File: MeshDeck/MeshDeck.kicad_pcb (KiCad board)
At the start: 4 copper layers, 44 parts, among them CN1 ATGM336H-6N-74, SW1 4*4*1.7, SW2 4*4*1.7, U1 ESP32-S3-WROOM-1(N16R8), U2 SX1262S8S+T-X1, U3 TPS6282533DMQR, U4 BQ24074RGTR, U5 RN32768114

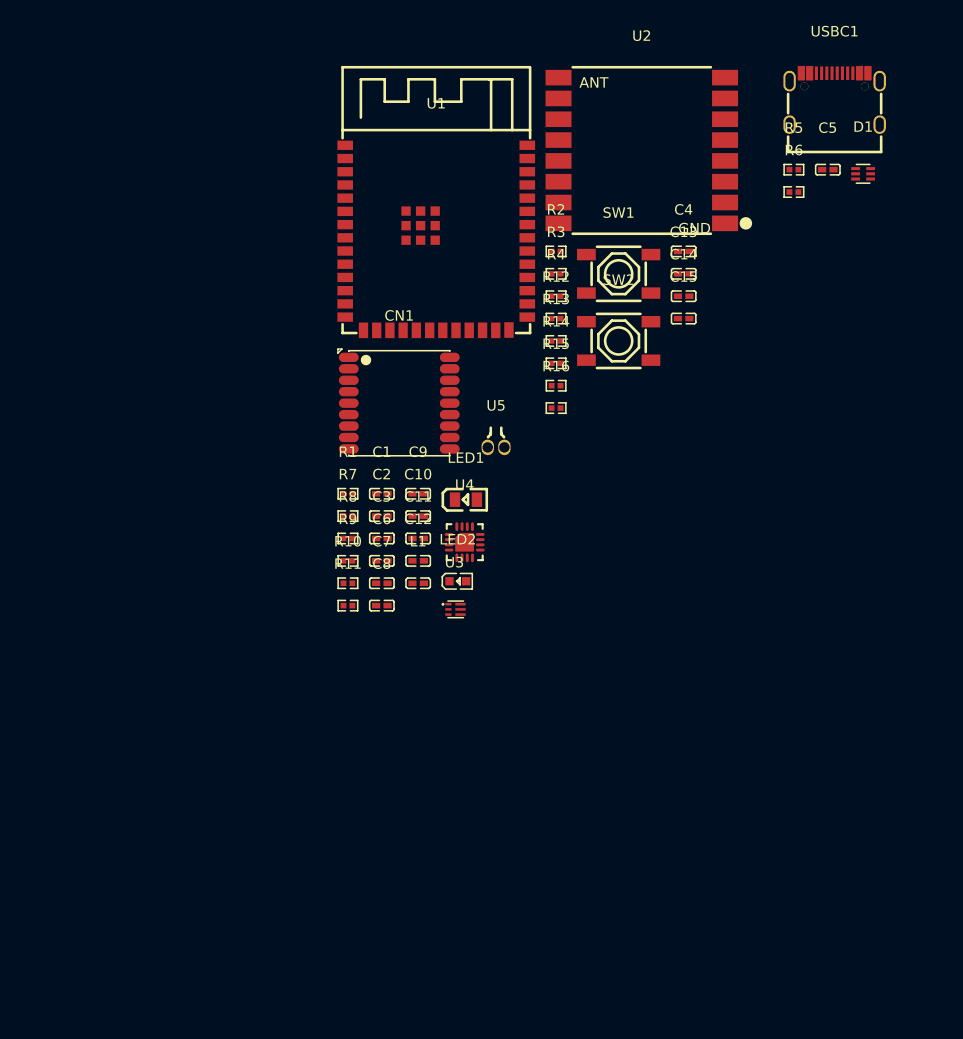
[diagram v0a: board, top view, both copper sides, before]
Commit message: set up LoRa module and screen (wip)
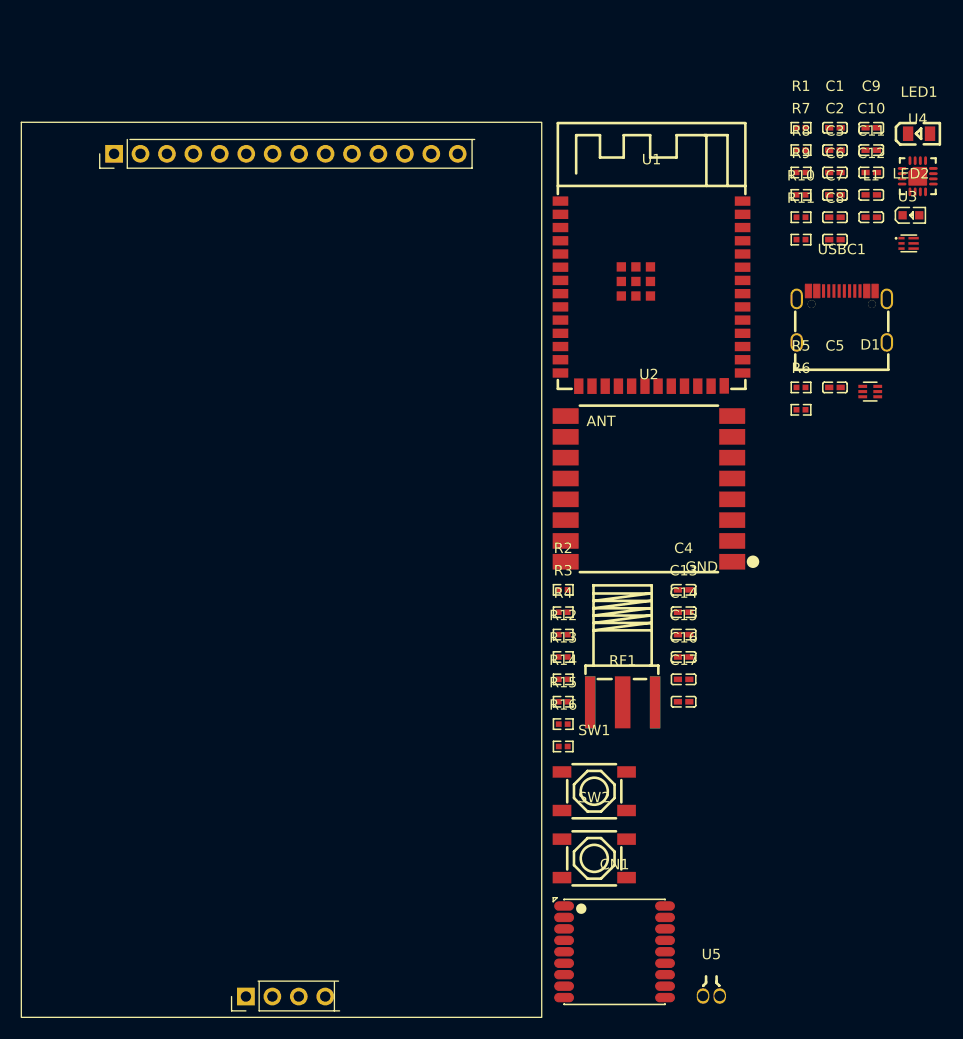
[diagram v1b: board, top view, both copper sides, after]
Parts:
- added C16: 1uF, MeshDeck:C0402, F.Cu at (153.0, 102.6)
- added C17: 1Nf, MeshDeck:C0402, F.Cu at (153.0, 104.7)
- added RF1: HJ-SMA023, MeshDeck:SMA-SMD_HJ-SMA023, F.Cu at (147.2, 104.8)
- added U6: ~, MeshDeck:2.8 SPI LCD TFT ST7789, F.Cu at (114.4, 69.3)
- moved U5 56.6 mm to (155.7, 133.0)
- moved CN1 56.6 mm to (146.4, 128.8)
- moved U3 56.0 mm to (174.6, 60.7)
- moved C11 56.0 mm to (171.1, 53.9)
- moved L1 56.0 mm to (171.1, 58.2)
- moved LED2 56.0 mm to (174.9, 58.0)
- moved R10 56.0 mm to (164.3, 58.2)
- moved R8 56.0 mm to (164.3, 53.9)
- moved U4 56.0 mm to (175.5, 54.2)
- moved C10 56.0 mm to (171.1, 51.7)
- moved C12 56.0 mm to (171.1, 56.0)
- moved C3 56.0 mm to (167.6, 53.9)
- moved C7 56.0 mm to (167.6, 58.2)
- moved C9 56.0 mm to (171.1, 49.6)
- moved LED1 56.0 mm to (175.7, 50.1)
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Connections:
- U1 pad 10: unconnected-(U1-IO17-Pad10) -> /IO17
- U1 pad 17: unconnected-(U1-IO9-Pad17) -> /IO9
- U1 pad 19: unconnected-(U1-IO11-Pad19) -> /IO11
- U1 pad 20: unconnected-(U1-IO12-Pad20) -> /IO12
- U1 pad 21: unconnected-(U1-IO13-Pad21) -> /IO13
- U1 pad 22: unconnected-(U1-IO14-Pad22) -> /IO14
- U1 pad 26: unconnected-(U1-IO45-Pad26) -> /IO45
- U1 pad 32: unconnected-(U1-IO39-Pad32) -> /SPI.SCK
- U1 pad 33: unconnected-(U1-IO40-Pad33) -> /SPI.MISO
- U1 pad 34: unconnected-(U1-IO41-Pad34) -> /SPI.MOSI
- U1 pad 35: unconnected-(U1-IO42-Pad35) -> /IO42
- U2 pad 1: unconnected-(U2-GND-Pad1) -> GND
- U2 pad 10: unconnected-(U2-GND-Pad10) -> GND
- U2 pad 11: unconnected-(U2-RXE-Pad11) -> /IO14
- U2 pad 13: unconnected-(U2-VCC-Pad13) -> /3V3
- U2 pad 15: unconnected-(U2-DIO1-Pad15) -> /IO45
- U2 pad 16: unconnected-(U2-BUSY-Pad16) -> /IO13
- U2 pad 2: unconnected-(U2-SO-Pad2) -> /SPI.MISO
- U2 pad 3: unconnected-(U2-SI-Pad3) -> /SPI.MOSI
- U2 pad 4: unconnected-(U2-SCK-Pad4) -> /SPI.SCK
- U2 pad 5: unconnected-(U2-NSS-Pad5) -> /IO9
- U2 pad 6: unconnected-(U2-RST-Pad6) -> /IO17
- U2 pad 8: unconnected-(U2-GND-Pad8) -> GND
- U2 pad 9: unconnected-(U2-ANT-Pad9) -> Net-(RF1-SIG)
